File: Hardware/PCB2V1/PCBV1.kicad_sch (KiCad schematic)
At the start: 21 parts, among them J1 Conn_02x07_Odd_Even, J2 Conn_01x03, J3 Conn_01x03, J4 Conn_01x08, SW1 SW_Push, U1 STM32L412KBTx

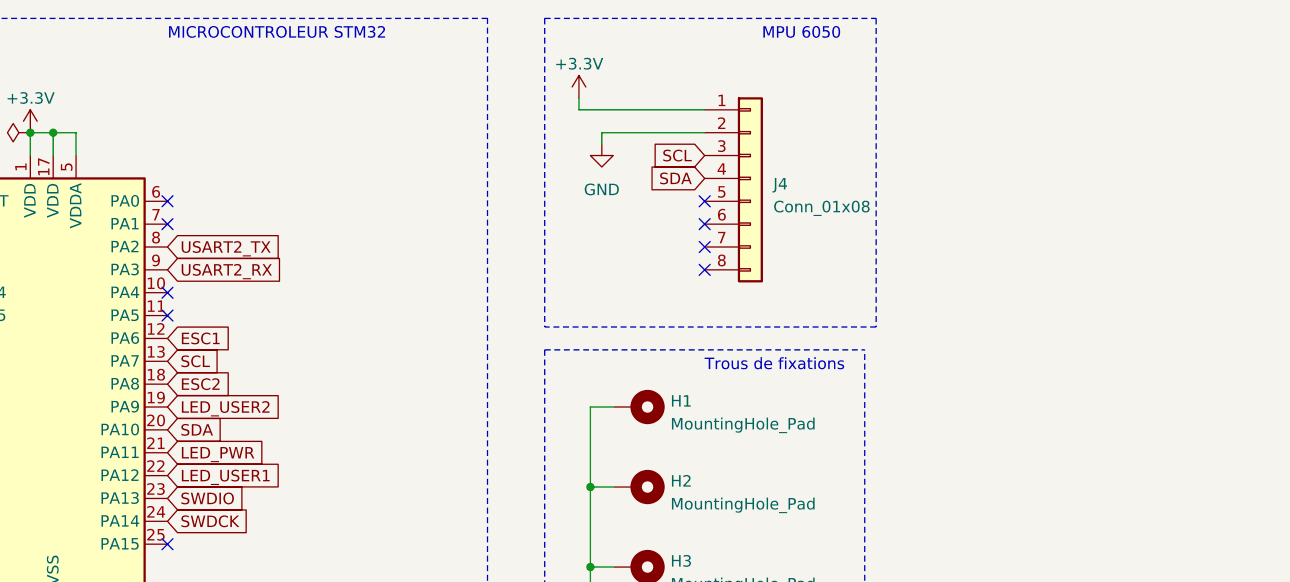
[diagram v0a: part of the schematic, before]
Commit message: message
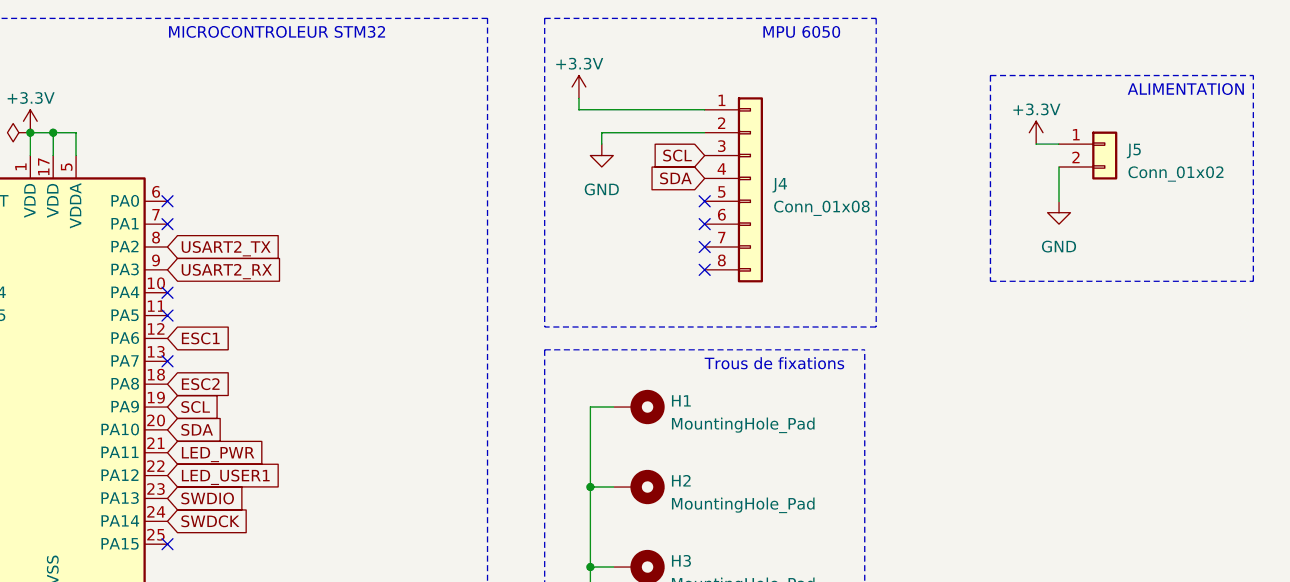
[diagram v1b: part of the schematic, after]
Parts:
- added J5: Conn_01x02, Connector_JST:JST_XH_B2B-XH-A_1x02_P2.50mm_Vertical, symbol Connector_Generic:Conn_01x02
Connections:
- net +3.3V: now also J5.1 (Pin_1)
- net GND: now also J5.2 (Pin_2)
- net LED_USER2: no longer U1.19 (PA9)
- net SCL: now also U1.19 (PA9); no longer U1.13 (PA7)
- no-connect marks 24 -> 25
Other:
- note added: "ALIMENTATION"
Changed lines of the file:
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@@
   (no_connect (at 102.87 128.27))
   (no_connect (at 52.07 63.5))
+  (no_connect (at 77.47 53.34))
   (no_connect (at 137.16 40.64))
   (no_connect (at 52.07 45.72))
@@
     (stroke (width 0) (type dash))
   )
+  (polyline (pts (xy 198.12 44.45) (xy 198.12 21.59))
+    (stroke (width 0) (type dash))
+  )
   (polyline (pts (xy 16.51 15.24) (xy 16.51 22.86))
     (stroke (width 0) (type dash))
@@
     (stroke (width 0) (type dash))
   )
+  (polyline (pts (xy 168.91 21.59) (xy 168.91 44.45))
+    (stroke (width 0) (type dash))
+  )
   (polyline (pts (xy 156.21 49.53) (xy 119.38 49.53))
     (stroke (width 0) (type dash))
@@
     (stroke (width 0) (type default))
   )
+  (polyline (pts (xy 168.91 44.45) (xy 198.12 44.45))
+    (stroke (width 0) (type dash))
+  )
   (wire (pts (xy 35.56 20.32) (xy 46.99 20.32))
     (stroke (width 0) (type default))
@@
     (stroke (width 0) (type default))
   )
+  (wire (pts (xy 173.99 29.21) (xy 176.53 29.21))
+    (stroke (width 0) (type default))
+  )
   (wire (pts (xy 24.13 121.92) (xy 29.21 121.92))
     (stroke (width 0) (type default))
@@
     (stroke (width 0) (type dash))
   )
+  (polyline (pts (xy 168.91 21.59) (xy 198.12 21.59))
+    (stroke (width 0) (type dash))
+  )
   (wire (pts (xy 87.63 123.19) (xy 87.63 120.65))
     (stroke (width 0) (type default))
@@
   )
   (wire (pts (xy 125.73 27.94) (xy 137.16 27.94))
+    (stroke (width 0) (type default))
+  )
+  (wire (pts (xy 176.53 35.56) (xy 176.53 31.75))
     (stroke (width 0) (type default))
   )
@@
   )
   (text "Trous de fixations" (at 137.16 54.61 0)
+    (effects (font (size 1.27 1.27)) (justify left bottom))
+  )
+  (text "ALIMENTATION" (at 184.15 24.13 0)
     (effects (font (size 1.27 1.27)) (justify left bottom))
   )
@@
     )
   )
-  (global_label "SCL" (shape input) (at 77.47 53.34 0) (fields_autoplaced)
-    (effects (font (size 1.27 1.27)) (justify left))
-    (property "Intersheetrefs" "${INTERSHEET_REFS}" (at 83.8834 53.34 0)
-      (effects (font (size 1.27 1.27)) (justify left) hide)
-    )
-  )
   (global_label "ESC2" (shape input) (at 102.87 125.73 180) (fields_autoplaced)
     (effects (font (size 1.27 1.27)) (justify right))
@@
     )
   )
-  (global_label "LED_USER2" (shape input) (at 77.47 58.42 0) (fields_autoplaced)
-    (effects (font (size 1.27 1.27)) (justify left))
-    (property "Intersheetrefs" "${INTERSHEET_REFS}" (at 90.959 58.42 0)
-      (effects (font (size 1.27 1.27)) (justify left) hide)
-    )
-  )
   (global_label "USART2_RX" (shape input) (at 77.47 43.18 0) (fields_autoplaced)
     (effects (font (size 1.27 1.27)) (justify left))
@@
     )
   )
+  (global_label "SCL" (shape input) (at 77.47 58.42 0) (fields_autoplaced)
+    (effects (font (size 1.27 1.27)) (justify left))
+    (property "Intersheetrefs" "${INTERSHEET_REFS}" (at 83.8834 58.42 0)
+      (effects (font (size 1.27 1.27)) (justify left) hide)
+    )
+  )
   (global_label "ESC1" (shape input) (at 77.47 50.8 0) (fields_autoplaced)
     (effects (font (size 1.27 1.27)) (justify left))
@@
         (path "/6a1fa79b-29e8-4816-8d7e-fabfcde671cf"
           (reference "#PWR05") (unit 1)
+        )
+      )
+    )
+  )
+  (symbol (lib_id "Connector_Generic:Conn_01x02") (at 181.61 29.21 0) (unit 1)
+    (in_bom yes) (on_board yes) (dnp no) (fields_autoplaced)
+    (property "Reference" "J5" (at 184.15 29.845 0)
+      (effects (font (size 1.27 1.27)) (justify left))
+    )
+    (property "Value" "Conn_01x02" (at 184.15 32.385 0)
+      (effects (font (size 1.27 1.27)) (justify left))
+    )
+    (property "Footprint" "Connector_JST:JST_XH_B2B-XH-A_1x02_P2.50mm_Vertical" (at 181.61 29.21 0)
+      (effects (font (size 1.27 1.27)) hide)
+    )
+    (property "Datasheet" "~" (at 181.61 29.21 0)
+      (effects (font (size 1.27 1.27)) hide)
+    )
+    (pin "1")
+    (pin "2")
+    (instances
+      (project "PCBV1"
+        (path "/1287c61c-3554-429d-9b6f-d3d4afb75d5d"
+          (reference "J5") (unit 1)
         )
       )
@@
         (path "/6a1fa79b-29e8-4816-8d7e-fabfcde671cf"
           (reference "C5") (unit 1)
+        )
+      )
+    )
+  )
+  (symbol (lib_id "power:+3.3V") (at 173.99 29.21 0) (unit 1)
+    (in_bom yes) (on_board yes) (dnp no) (fields_autoplaced)
+    (property "Reference" "#PWR020" (at 173.99 33.02 0)
+      (effects (font (size 1.27 1.27)) hide)
+    )
+    (property "Value" "+3.3V" (at 173.99 25.4 0)
+      (effects (font (size 1.27 1.27)))
+    )
+    (property "Footprint" "" (at 173.99 29.21 0)
+      (effects (font (size 1.27 1.27)) hide)
+    )
+    (property "Datasheet" "" (at 173.99 29.21 0)
+      (effects (font (size 1.27 1.27)) hide)
+    )
+    (pin "1")
+    (instances
+      (project "PCBV1"
+        (path "/1287c61c-3554-429d-9b6f-d3d4afb75d5d"
+          (reference "#PWR020") (unit 1)
+        )
+      )
+      (project "Schema_alimentation"
+        (path "/6a1fa79b-29e8-4816-8d7e-fabfcde671cf"
+          (reference "#PWR09") (unit 1)
         )
       )
@@
         )
       )
+    )
+  )
+  (symbol (lib_id "power:GND") (at 176.53 35.56 0) (unit 1)
+    (in_bom yes) (on_board yes) (dnp no) (fields_autoplaced)
+    (property "Reference" "#PWR019" (at 176.53 41.91 0)
+      (effects (font (size 1.27 1.27)) hide)
+    )
+    (property "Value" "GND" (at 176.53 40.64 0)
+      (effects (font (size 1.27 1.27)))
+    )
+    (property "Footprint" "" (at 176.53 35.56 0)
+      (effects (font (size 1.27 1.27)) hide)
+    )
+    (property "Datasheet" "" (at 176.53 35.56 0)
+      (effects (font (size 1.27 1.27)) hide)
+    )
+    (pin "1")
+    (instances
+      (project "PCBV1"
+        (path "/1287c61c-3554-429d-9b6f-d3d4afb75d5d"
+          (reference "#PWR019") (unit 1)
+        )
+      )
+      (project "Schema_alimentation"
+        (path "/6a1fa79b-29e8-4816-8d7e-fabfcde671cf"
+          (reference "#PWR014") (unit 1)
+        )
+      )
